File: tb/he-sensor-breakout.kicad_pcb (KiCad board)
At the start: 2 copper layers, 19.1 x 29.1 mm, 35 parts, among them J1 Conn_01x01_Pin, J10 Conn_01x01_Pin, J11 Conn_01x01_Pin, J12 Conn_01x01_Pin, J13 Conn_01x01_Pin, J14 Conn_01x01_Pin, J2 Conn_01x01_Pin, J3 Conn_01x01_Pin, J4 Conn_01x01_Pin, J5 Conn_01x01_Pin, J6 Conn_01x01_Pin, J7 Conn_01x01_Pin, J8 Conn_01x01_Pin, J9 Conn_01x01_Pin, U1 SLSS49E

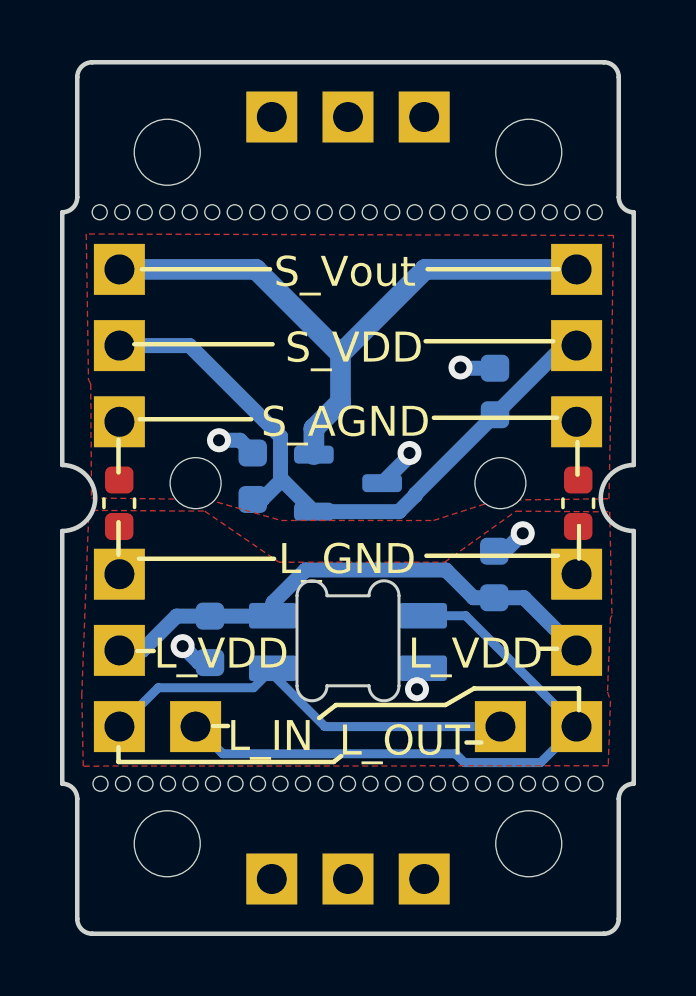
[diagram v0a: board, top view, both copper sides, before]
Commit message: finishing touches
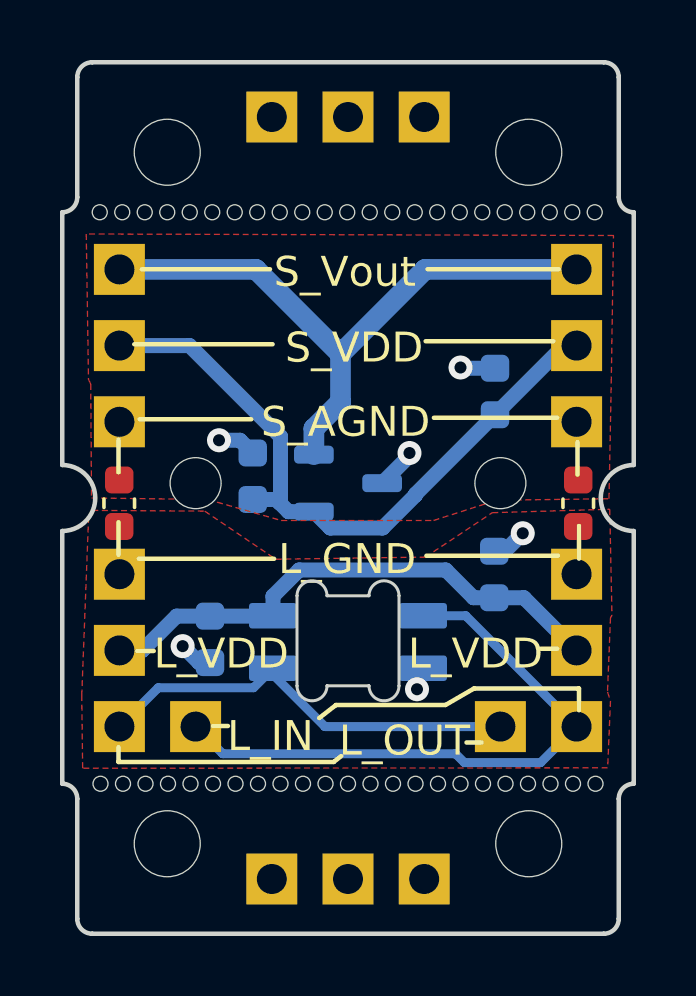
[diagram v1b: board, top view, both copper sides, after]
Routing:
- net VDDA: track 22.3 -> 23.0 mm
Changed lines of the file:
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@@
   (segment (start 102.05 98.5) (end 102.05 98.592933) (width 0.5) (layer "B.Cu") (net 1))
   (segment (start 92.82 94.92) (end 92.38 94.92) (width 0.5) (layer "F.Cu") (net 2))
+  (segment (start 97.75 97.95) (end 97.75 100.13) (width 0.5) (layer "B.Cu") (net 2))
+  (segment (start 102.25 99.903961) (end 101.153961 101) (width 0.5) (layer "B.Cu") (net 2))
+  (segment (start 99.407067 101) (end 98.8625 100.455433) (width 0.5) (layer "B.Cu") (net 2))
+  (segment (start 94.72 94.92) (end 97.75 97.95) (width 0.5) (layer "B.Cu") (net 2))
+  (segment (start 101.153961 101) (end 99.407067 101) (width 0.5) (layer "B.Cu") (net 2))
+  (segment (start 102.25 99.875) (end 102.25 99.903961) (width 0.5) (layer "B.Cu") (net 2))
+  (segment (start 98.015433 100.455433) (end 97.72 100.16) (width 0.5) (layer "B.Cu") (net 2))
+  (segment (start 97.75 100.13) (end 97.72 100.16) (width 0.5) (layer "B.Cu") (net 2))
+  (segment (start 98.8625 100.455433) (end 98.015433 100.455433) (width 0.5) (layer "B.Cu") (net 2))
   (segment (start 107.205 94.92) (end 102.25 99.875) (width 0.5) (layer "B.Cu") (net 2))
+  (segment (start 96.825 100.05) (end 97.61 100.05) (width 0.5) (layer "B.Cu") (net 2))
+  (segment (start 97.61 100.05) (end 97.72 100.16) (width 0.5) (layer "B.Cu") (net 2))
   (segment (start 92.38 94.92) (end 94.72 94.92) (width 0.5) (layer "B.Cu") (net 2))
-  (segment (start 97.75 99.436683) (end 97.84375 99.436683) (width 0.5) (layer "B.Cu") (net 2))
-  (segment (start 102.25 99.903961) (end 101.698528 100.455433) (width 0.5) (layer "B.Cu") (net 2))
-  (segment (start 101.698528 100.455433) (end 98.8625 100.455433) (width 0.5) (layer "B.Cu") (net 2))
-  (segment (start 97.84375 99.436683) (end 98.8625 100.455433) (width 0.5) (layer "B.Cu") (net 2))
-  (segment (start 97.75 97.95) (end 97.75 99.436683) (width 0.5) (layer "B.Cu") (net 2))
-  (segment (start 94.72 94.92) (end 97.75 97.95) (width 0.5) (layer "B.Cu") (net 2))
-  (segment (start 97.75 99.436683) (end 97.136683 100.05) (width 0.5) (layer "B.Cu") (net 2))
-  (segment (start 102.25 99.875) (end 102.25 99.903961) (width 0.5) (layer "B.Cu") (net 2))
   (segment (start 107.62 94.92) (end 107.205 94.92) (width 0.5) (layer "B.Cu") (net 2))
-  (segment (start 97.136683 100.05) (end 96.825 100.05) (width 0.5) (layer "B.Cu") (net 2))
   (via (at 94.488188 104.938188) (size 0.8) (drill 0.4) (layers "F.Cu" "B.Cu") (free) (net 3))
   (via (at 102.3 106.375) (size 0.8) (drill 0.4) (layers "F.Cu" "B.Cu") (free) (net 3))
@@
   (segment (start 105.225 101.775) (end 105.825 101.175) (width 0.5) (layer "B.Cu") (net 3))
   (segment (start 94.288317 103.936683) (end 95.4 103.936683) (width 0.5) (layer "B.Cu") (net 4))
-  (segment (start 97.5 103.487664) (end 97.5 103.925) (width 0.5) (layer "B.Cu") (net 4))
+  (segment (start 98.37 102.4) (end 97.5 103.27) (width 0.5) (layer "B.Cu") (net 4))
   (segment (start 93.145 105.08) (end 94.288317 103.936683) (width 0.5) (layer "B.Cu") (net 4))
   (segment (start 95.4 103.936683) (end 97.488317 103.936683) (width 0.5) (layer "B.Cu") (net 4))
+  (segment (start 97.5 103.27) (end 97.5 103.925) (width 0.5) (layer "B.Cu") (net 4))
+  (segment (start 105.865 103.325) (end 104.185051 103.325) (width 0.5) (layer "B.Cu") (net 4))
+  (segment (start 97.488317 103.936683) (end 97.5 103.925) (width 0.5) (layer "B.Cu") (net 4))
   (segment (start 107.62 105.08) (end 105.865 103.325) (width 0.5) (layer "B.Cu") (net 4))
-  (segment (start 98.587664 102.4) (end 97.5 103.487664) (width 0.5) (layer "B.Cu") (net 4))
-  (segment (start 97.488317 103.936683) (end 97.5 103.925) (width 0.5) (layer "B.Cu") (net 4))
-  (segment (start 105.865 103.325) (end 104.185051 103.325) (width 0.5) (layer "B.Cu") (net 4))
-  (segment (start 103.260051 102.4) (end 98.587664 102.4) (width 0.5) (layer "B.Cu") (net 4))
   (segment (start 104.185051 103.325) (end 103.260051 102.4) (width 0.5) (layer "B.Cu") (net 4))
+  (segment (start 103.260051 102.4) (end 98.37 102.4) (width 0.5) (layer "B.Cu") (net 4))
   (segment (start 92.38 105.08) (end 93.145 105.08) (width 0.5) (layer "B.Cu") (net 4))
   (segment (start 95.825 108.525) (end 94.92 107.62) (width 0.3) (layer "B.Cu") (net 5))
@@
         (xy 91.474749 100.412665)
         (xy 95.224749 100.437665)
-        (xy 97.699749 102.137665)
-        (xy 103.224749 102.137665)
-        (xy 105.599749 100.437665)
-        (xy 108.724749 100.462665)
+        (xy 97.59 102.04)
+        (xy 102.58 101.97)
+        (xy 104.81 100.49)
+        (xy 108.724749 100.375)
         (xy 108.799749 103.912665)
         (xy 108.749749 103.987665)
         (xy 108.649749 106.462665)
         (xy 108.749749 106.762665)
-        (xy 108.675 108.925)
-        (xy 91.175 108.937665)
+        (xy 108.655 108.995)
+        (xy 91.155 109.007665)
         (xy 91.124749 106.587665)
         (xy 91.35 100.725)
